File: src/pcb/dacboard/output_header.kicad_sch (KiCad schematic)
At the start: 1 part, among them J3 Conn_01x24_Socket

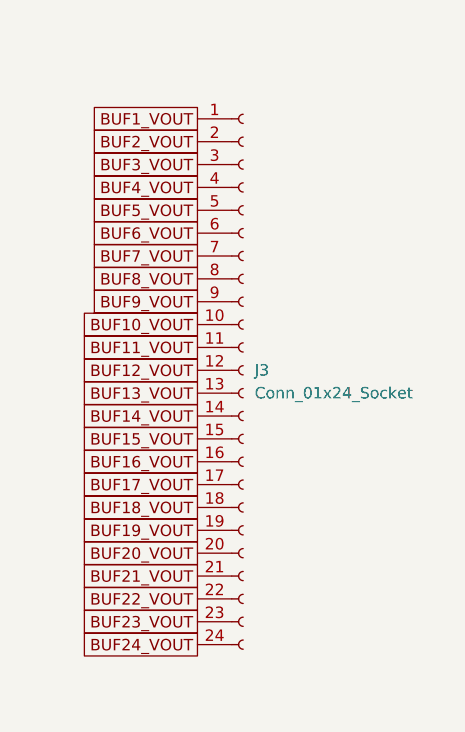
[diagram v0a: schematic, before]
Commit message: dacboard routing
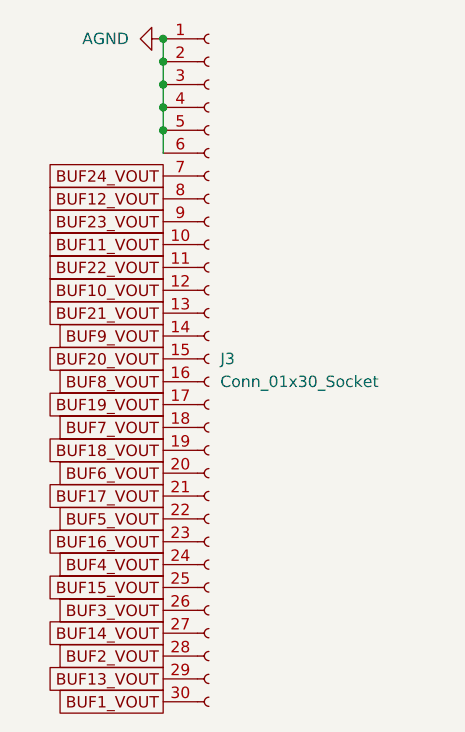
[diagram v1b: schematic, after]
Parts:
- removed J3: Conn_01x24_Socket, symbol Connector:Conn_01x24_Socket
- added J3: Conn_01x30_Socket, Connector_PinHeader_2.54mm:PinHeader_1x30_P2.54mm_Horizontal, symbol Connector:Conn_01x30_Socket
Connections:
- net BUF10_VOUT: now also J3.12 (Pin_12)
- net BUF11_VOUT: now also J3.10 (Pin_10)
- net BUF12_VOUT: now also J3.8 (Pin_8)
- net BUF13_VOUT: now also J3.29 (Pin_29)
- net BUF14_VOUT: now also J3.27 (Pin_27)
- net BUF15_VOUT: now also J3.25 (Pin_25)
- net BUF16_VOUT: now also J3.23 (Pin_23)
- net BUF17_VOUT: now also J3.21 (Pin_21)
- net BUF18_VOUT: now also J3.19 (Pin_19)
- net BUF19_VOUT: now also J3.17 (Pin_17)
- net BUF1_VOUT: now also J3.30 (Pin_30)
- net BUF20_VOUT: now also J3.15 (Pin_15)
- net BUF21_VOUT: now also J3.13 (Pin_13)
- net BUF22_VOUT: now also J3.11 (Pin_11)
- net BUF23_VOUT: now also J3.9 (Pin_9)
- net BUF24_VOUT: now also J3.7 (Pin_7)
- net BUF2_VOUT: now also J3.28 (Pin_28)
- net BUF3_VOUT: now also J3.26 (Pin_26)
- net BUF4_VOUT: now also J3.24 (Pin_24)
- net BUF5_VOUT: now also J3.22 (Pin_22)
- net BUF6_VOUT: now also J3.20 (Pin_20)
- net BUF7_VOUT: now also J3.18 (Pin_18)
- net BUF8_VOUT: now also J3.16 (Pin_16)
- net BUF9_VOUT: now also J3.14 (Pin_14)
- new net AGND: J3.1 (Pin_1), J3.2 (Pin_2), J3.3 (Pin_3), J3.4 (Pin_4), J3.5 (Pin_5), J3.6 (Pin_6)
